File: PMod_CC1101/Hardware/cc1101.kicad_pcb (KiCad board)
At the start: 2 copper layers, 16 parts, among them J1 Conn_Coaxial, J2 Conn_02x06_Odd_Even

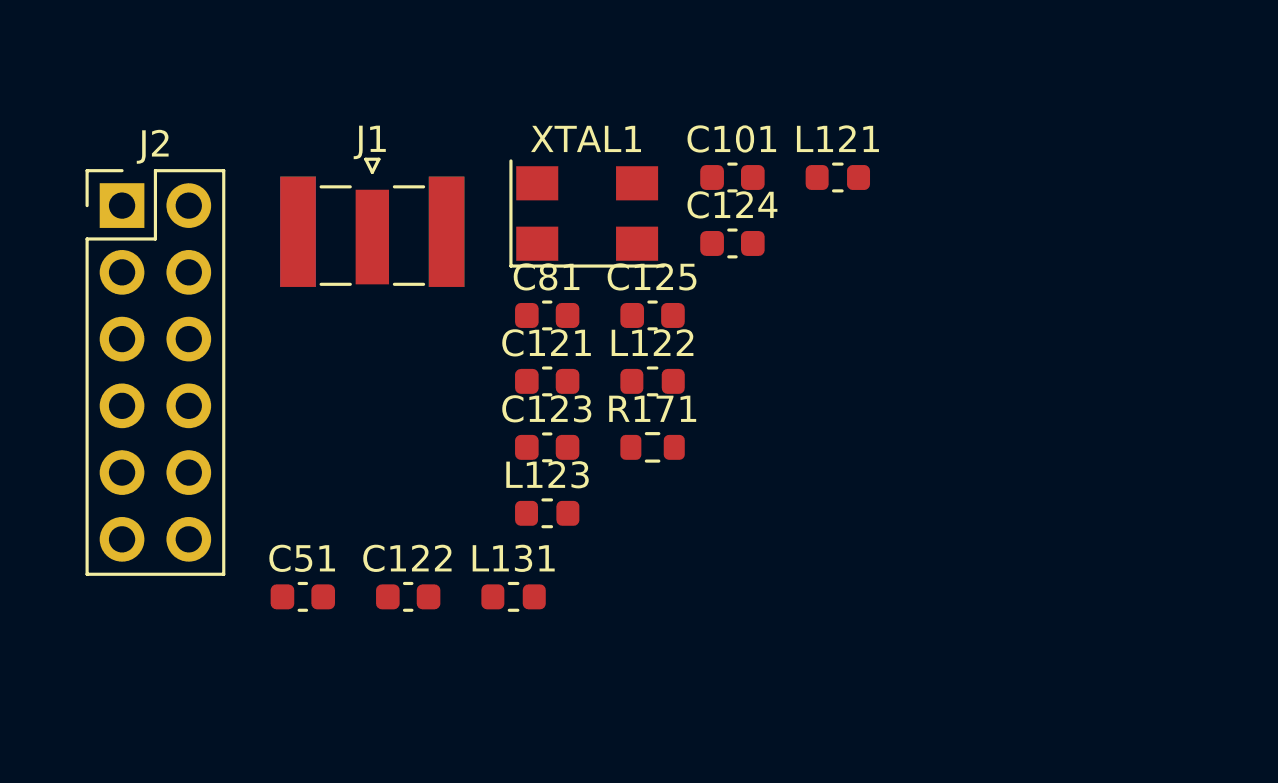
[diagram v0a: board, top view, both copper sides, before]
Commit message: initial footprint for the CC1101 part
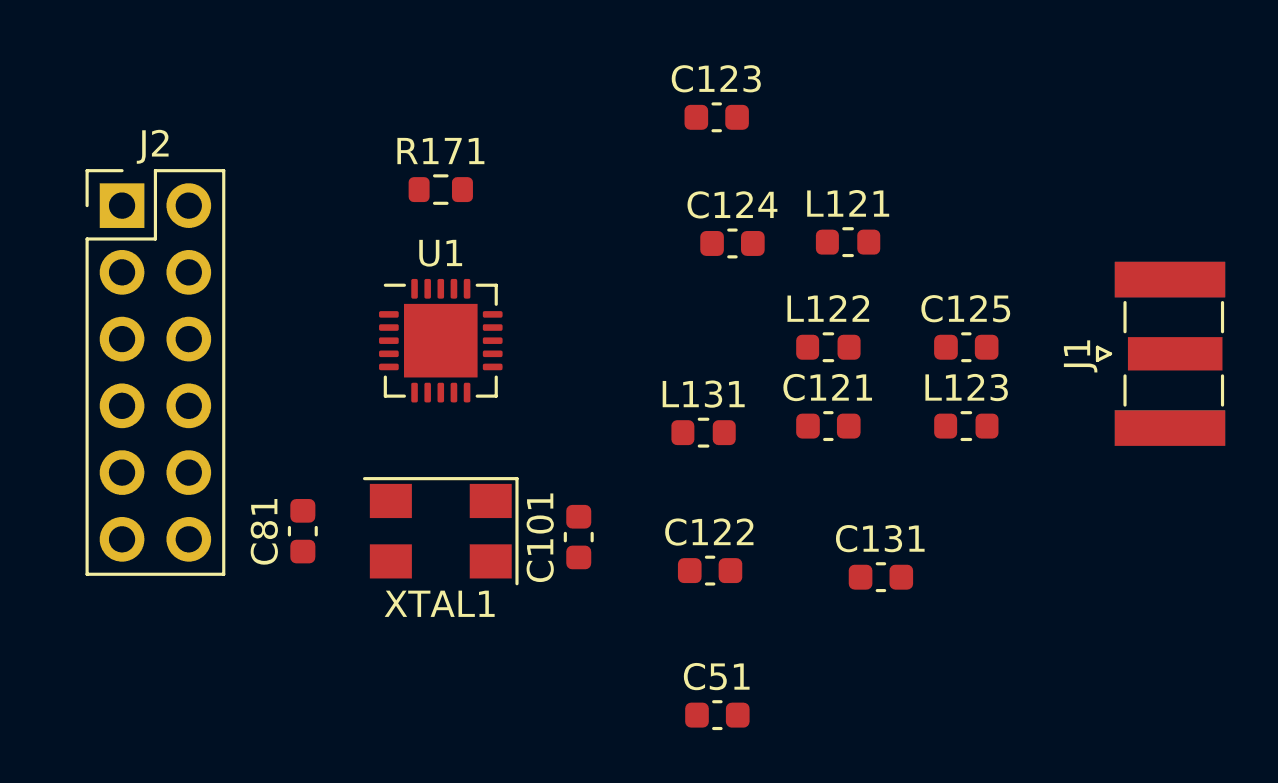
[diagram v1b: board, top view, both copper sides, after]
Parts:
- added C131: 3.9pF, Capacitor_SMD:C_0603_1608Metric, F.Cu at (162.5, 70.8)
- added U1: CC1101RGPR, Package_DFN_QFN:UQFN-20-1EP_4x4mm_P0.5mm_EP2.8x2.8mm, F.Cu at (145.8, 61.8)
- moved J1 30.7 mm to (173.5, 62.2), turned to 90 degrees
- moved C51 16.4 mm to (156.3, 76.0)
- moved L123 16.3 mm to (165.8, 65.0)
- moved C101 14.9 mm to (151.0, 69.2), turned to 90 degrees
- moved C123 14.1 mm to (156.2, 53.2)
- moved XTAL1 13.3 mm to (145.8, 69.0), turned to 180 degrees
- moved R171 12.7 mm to (145.8, 56.0)
- moved C81 12.4 mm to (140.5, 69.0), turned to 90 degrees
- moved C125 12.0 mm to (165.8, 62.0)
- moved C122 11.5 mm to (156.0, 70.5)
- moved C121 10.8 mm to (160.5, 65.0)
- moved L131 9.56 mm to (155.8, 65.2)
- moved L122 6.82 mm to (160.5, 62.0)
- moved L121 2.49 mm to (161.2, 58.0)

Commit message: Component positioned within board edges
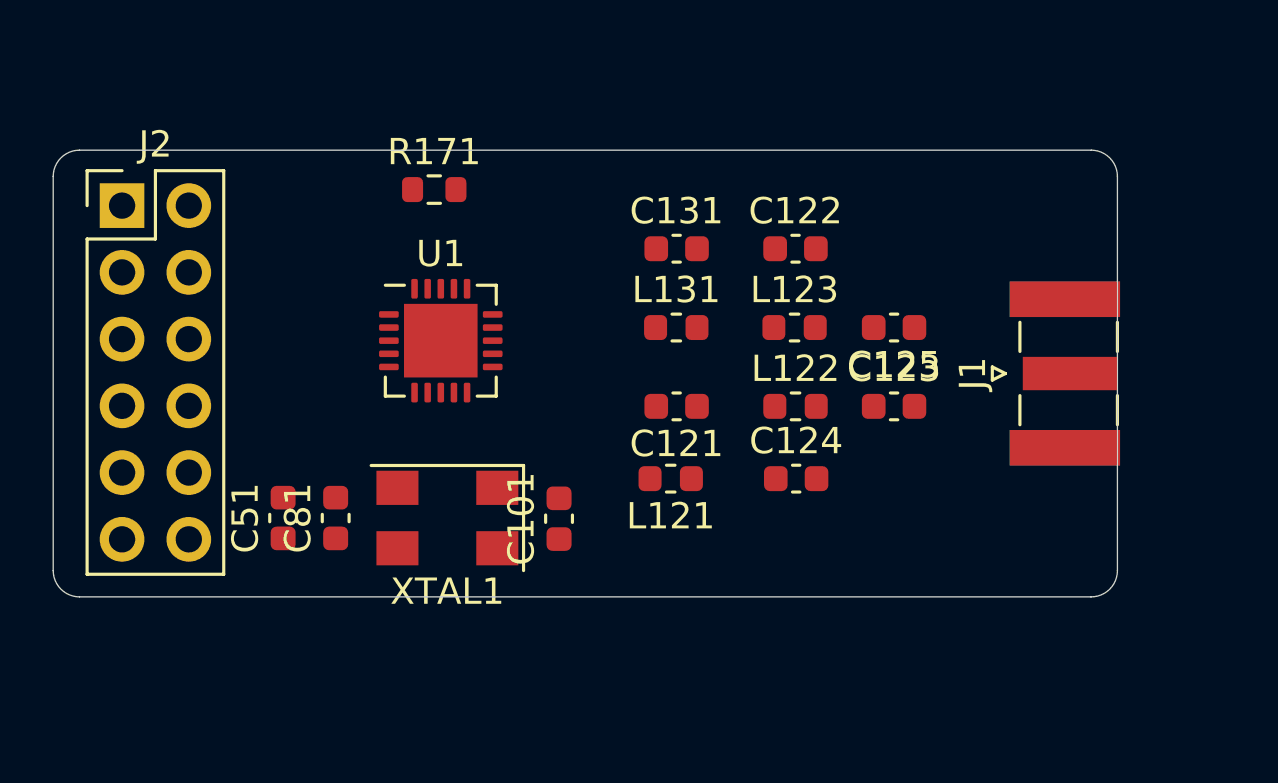
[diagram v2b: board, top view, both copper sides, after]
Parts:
- moved C51 18.1 mm to (139.8, 68.5), turned to 90 degrees
- moved C131 14.7 mm to (154.7, 58.2)
- moved C123 12.9 mm to (163.0, 64.2)
- moved C122 12.7 mm to (159.2, 58.2)
- moved L121 11.2 mm to (154.5, 67.0), turned to 180 degrees
- moved C124 9.27 mm to (159.3, 67.0)
- moved L123 7.54 mm to (159.2, 61.2)
- moved C121 5.82 mm to (154.7, 64.2), turned to 180 degrees
- moved L131 4.13 mm to (154.7, 61.2)
- moved J1 4.07 mm to (169.5, 63.0)
- moved C125 2.85 mm to (163.0, 61.2), turned to 180 degrees
- moved L122 2.57 mm to (159.2, 64.2)
- moved C81 1.35 mm to (141.8, 68.5)
- moved C101 1.03 mm to (150.2, 68.5)
- moved XTAL1 0.56 mm to (146.0, 68.5)
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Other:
- board outline added: 40.5 x 17 mm

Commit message: line up the RF componnents on the board
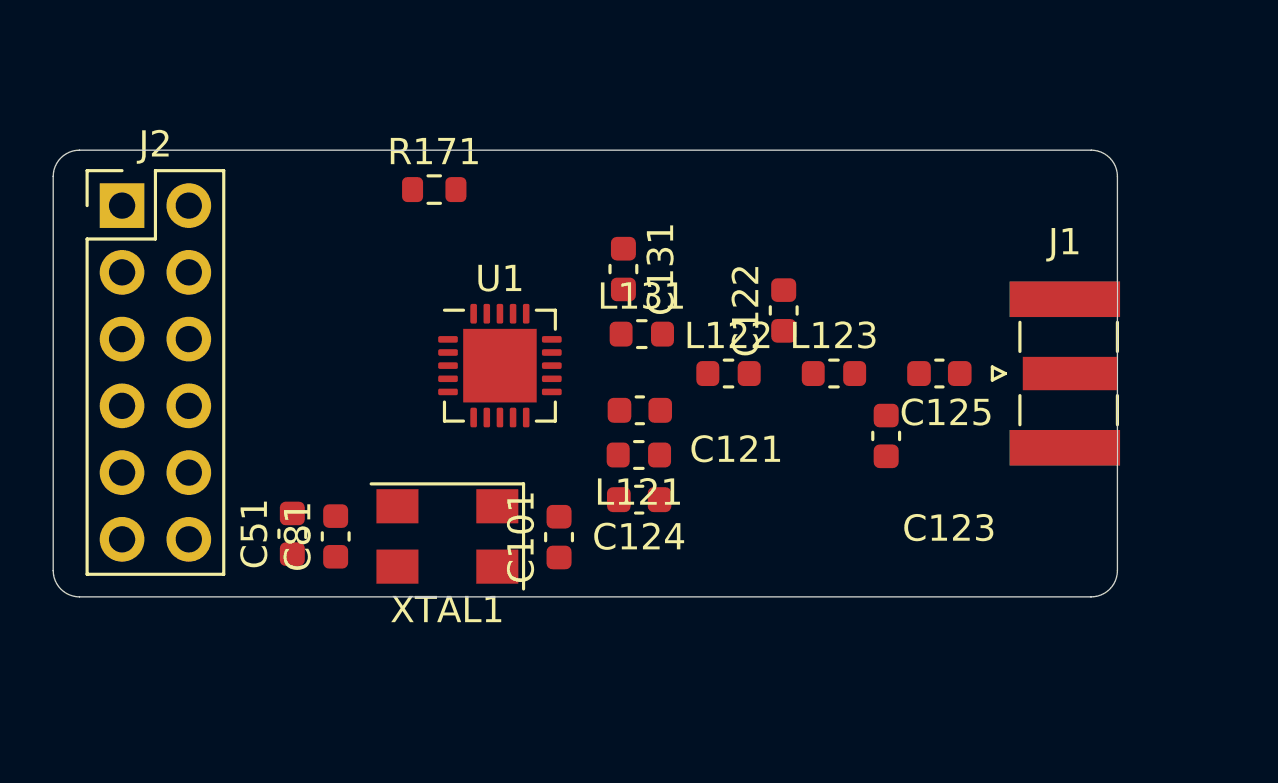
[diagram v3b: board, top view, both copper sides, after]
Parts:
- moved C124 6.03 mm to (153.3, 67.8), turned to 180 degrees
- moved L122 2.84 mm to (156.7, 63.0)
- moved C125 2.46 mm to (164.7, 63.0)
- moved U1 2.44 mm to (148.0, 62.7)
- moved C122 2.39 mm to (158.8, 60.6), turned to 90 degrees
- moved L123 2.30 mm to (160.7, 63.0)
- moved C131 2.17 mm to (152.7, 59.0), turned to 270 degrees
- moved L121 1.51 mm to (153.3, 66.1)
- moved C121 1.41 mm to (153.3, 64.4)
- moved L131 1.34 mm to (153.4, 61.5)
- moved C123 1.16 mm to (162.7, 65.4), turned to 270 degrees
- moved C81 0.70 mm to (141.8, 69.2)
- moved XTAL1 0.70 mm to (146.0, 69.2)
- moved C101 0.70 mm to (150.2, 69.2)
- moved C51 0.69 mm to (140.1, 69.1)
